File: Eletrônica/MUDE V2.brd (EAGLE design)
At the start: 35 x 16 mm, 36 parts, among them J1 22-05-7038-03, J2 22-05-7038-03, Q1 MOSFET-NCHANNEL2N7002PW, Q2 MOSFET-NCHANNEL2N7002PW, Q3 MOSFET-NCHANNEL2N7002PW, Q4 MOSFET-NCHANNEL2N7002PW, Q5 MOSFET-NCHANNEL2N7002PW, U2 Tiny85-20-SMT

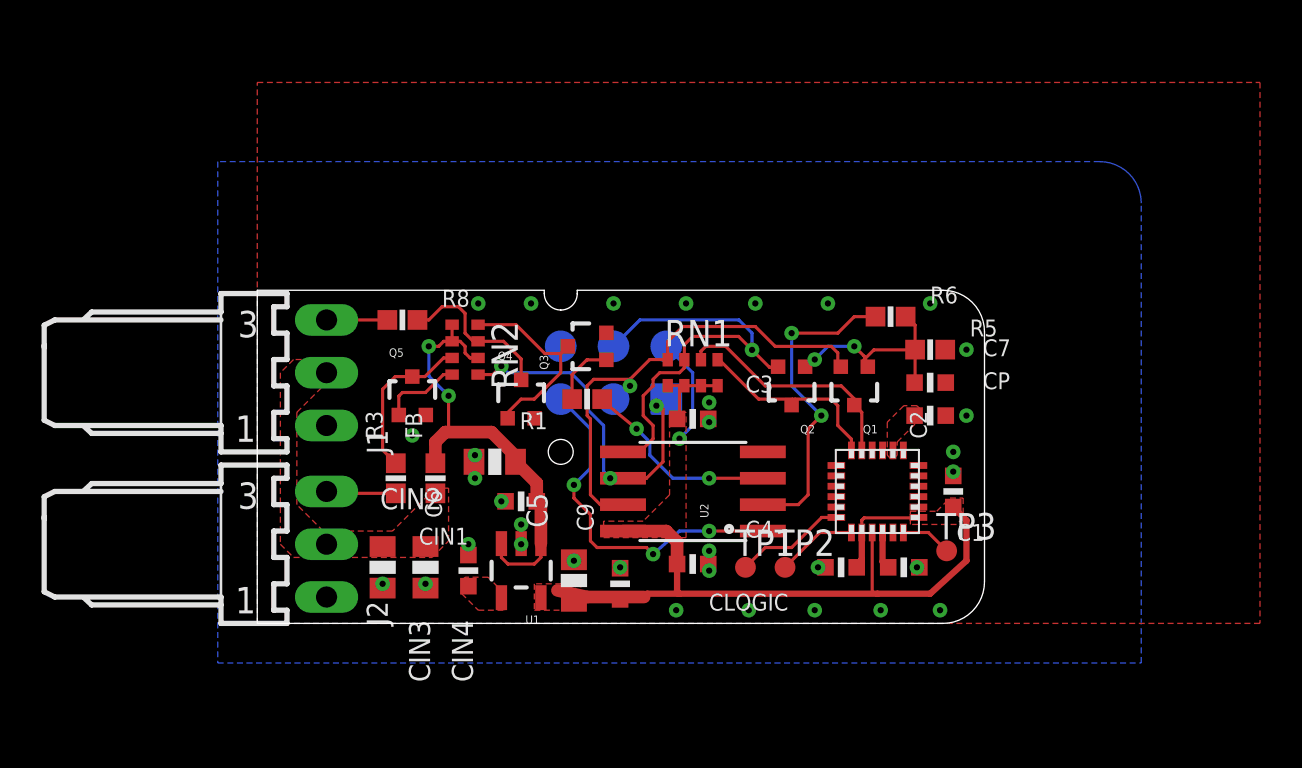
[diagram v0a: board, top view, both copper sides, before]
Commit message: MUDE V2 files
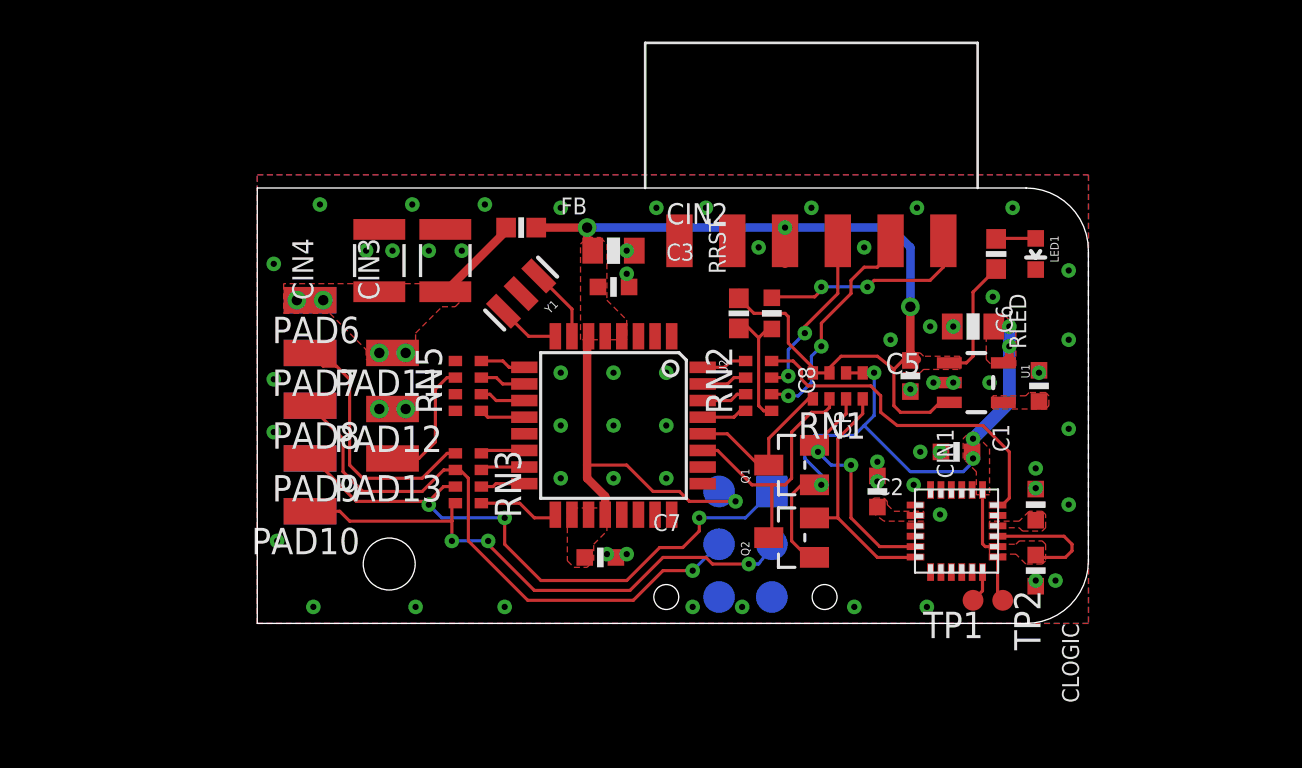
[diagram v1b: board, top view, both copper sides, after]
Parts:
- removed C4, C9: 1uF, wes:C0603
- removed J1, J2: 22-05-7038-03, con-molex:7395-03
- removed Q3, Q4, Q5: MOSFET-NCHANNEL2N7002PW, SparkFun-DiscreteSemi:SOT323
- removed R1, R3, R5, R6, R8: (no value), wes:R0603
- removed TP3: TPSQTP10R, testpad:TP10R
- added C8: 100nF, wes:C0603
- added LED1: (no value), SparkFun-LED:LED-0603
- added PAD1, PAD10, PAD11, PAD12, PAD13, PAD2, PAD3, PAD4, PAD5, PAD6, PAD7, PAD8, PAD9: (no value), wirepad:SMD1,27-2,54
- added RLED, RRST: (no value), wes:R0603
- added RN3, RN5: (no value), resistor-dil:0603-ARV
- added U$2: FTDI_HEADERSMD, wes:FTDI_HEADER_SMD
- added Y1: 16MHz, SparkFun-FreqCtrl:RESONATOR-SMD
- CIN3, CIN4: device wes:C0805 -> wes:C1210
- Q1, Q2: value MOSFET-NCHANNEL2N7002PW -> NFET; device SparkFun-DiscreteSemi:SOT323 -> SparkFun-DiscreteSemi:SOT23
- U$3: value ISP_POGOISP_LHOLE -> ISP_POGOISP_POGO; device wes:ISP_POGO_LHOLE -> wes:ISP_POGO
- U2: value Tiny85-20-SMT -> ATMEGA328P; device SparkFun-DigitalIC:SO08-EIAJ -> SparkFun-DigitalIC:TQFP32-08
- moved C6 28.9 mm to (37.6, 11.4)
- moved U1 23.7 mm to (34.6, 11.6), turned to 270 degrees
- moved C5 22.8 mm to (34.4, 14.3), turned to 180 degrees
- moved CIN1 19.7 mm to (31.4, 11.9), turned to 270 degrees
- moved C7 18.0 mm to (16.5, 3.17)
- moved CIN3 15.1 mm to (9.05, 17.5), turned to 90 degrees
- moved CIN4 14.9 mm to (5.87, 17.5), turned to 90 degrees
- moved RN2 14.2 mm to (24.1, 11.4), turned to 270 degrees
- moved FB 12.8 mm to (12.7, 19.1), turned to 0 degrees
- moved CIN2 11.7 mm to (17.1, 17.9), turned to 0 degrees
- moved TP1 11.1 mm to (34.4, 1.11), turned to 180 degrees
- moved TP2 10.6 mm to (35.9, 1.11), turned to 270 degrees
- moved U$3 10.4 mm to (23.5, 3.81), turned to 0 degrees
- moved CLOGIC 9.37 mm to (37.5, 2.54), turned to 270 degrees
- moved C3 7.41 mm to (17.1, 16.2)
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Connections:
- removed net ATTINYOUT: J2.3, R3.1
- removed net DATAOUT: R1.1, U2.3
- removed net I2C-SWITCH: R6.1, U2.2
- removed net N$17: C7.1, Q1.1, Q2.1, R5.1, R6.2
- removed net N$21: Q4.3, R8.2, RN2.3
- removed net SCL/SCK: Q1.2, RN1.4, U$3.SCK, U2.7
- removed net SDA/MOSI: Q2.2, RN1.3, U$3.MOSI, U2.5
- removed net VIN: CIN3.1, CIN4.1, FB.1, J1.2, J2.2
- new net +5V: C3.1, C7.1, CIN1.1, CIN2.1, FB.2, RLED.2, RN1.7, RN1.8, RRST.2, U$2.VCC, U$3.VCC, U1.1, U1.3, U2.18, U2.20, U2.4, U2.6
- new net DTR: C8.1, U$2.DTR
- new net MOSI: PAD8.1, RN3.6, U$3.MOSI
- new net MPU_INT: RN2.8, U$1.12
- new net N$10: U2.7, Y1.1
- new net N$15: U2.8, Y1.3
- new net N$19: RN2.4, U2.29
- new net N$20: RN5.6, U2.11
- new net N$22: RN3.1, U2.17
- new net N$23: RN3.2, U2.16
- new net N$24: RN3.3, U2.15
- new net N$25: RN3.4, U2.14
- new net N$26: RN5.5, U2.12
- new net N$29: C8.2, RN2.5, RRST.1
- new net N$30: RN5.1
- new net N$32: RN5.3
- new net N$33: RN5.4
- new net N$8: RN5.8, U2.9
- new net RX: RN2.6, U$2.RX
- new net SCK: PAD10.1, RN3.8, U$3.SCK
- new net SCL: Q1.3, RN1.1, U2.28
- new net SDA: Q2.3, RN1.2, U2.27
- new net SS: PAD7.1, RN3.5
- new net TX: RN2.7, U$2.TX
- net +3V3: now also Q1.1, Q2.1; no longer C3.1, C4.1, C9.1, RN1.7, RN1.8, U$3.VCC, U2.8
- net GND: now also LED1.C, PAD12.1, PAD2.1, PAD3.1, PAD4.1, PAD5.1, U$2.GND, U2.21, U2.3, U2.5, Y1.2; no longer C4.2, C9.2, J1.1, J2.1, Q3.2, Q4.2, Q5.2, R5.2, U2.4
- net MISO: now also PAD9.1, RN3.7; no longer RN2.1, U2.6
- net N$11: now also LED1.A, RLED.1; no longer TP3.TP, U$1.12
- net N$14: now also RN2.2, U2.31; no longer Q3.1, R1.2
- net N$16: now also RN5.7, U2.10; no longer Q3.3, Q4.1, RN2.4
- net N$18: now also RN2.1, U2.32; no longer Q5.3, R3.2, RN2.7
- net N$2: now also RN2.3, U2.30; no longer Q5.1, RN2.8
- net N$7: now also Q2.2, RN1.4; no longer Q2.3, RN1.1
- net N$9: now also Q1.2, RN1.3; no longer Q1.3, RN1.2
- net NEOPIXELS: now also PAD13.1, RN5.2; no longer J1.3, R8.1
- net RST: no longer U2.1
- net V+: now also CIN3.1, CIN4.1, FB.1, PAD1.1, PAD11.1, PAD6.1; no longer CIN1.1, CIN2.1, FB.2, RN2.2, RN2.5, RN2.6, U1.1, U1.3
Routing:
- net +5V: track 0.00 -> 68.6 mm, vias 0 -> 4
- net MOSI: track 0.00 -> 28.2 mm, vias 0 -> 1
- net SCK: track 0.00 -> 27.0 mm, vias 0 -> 3
- net SCL/SCK: track 23.7 -> 0.00 mm, vias 1 -> 0
- net SDA/MOSI: track 21.4 -> 0.00 mm, vias 1 -> 0
- net V+: track 22.1 -> 4.93 mm, vias 2 -> 4
- net RST: track 17.1 -> 0.00 mm, vias 3 -> 0
- net MPU_INT: track 0.00 -> 16.9 mm
- net I2C-SWITCH: track 15.4 -> 0.00 mm, vias 2 -> 0
- net SDA: track 0.00 -> 12.7 mm
- net SS: track 0.00 -> 12.4 mm
- net MISO: track 17.0 -> 29.2 mm
- net RX: track 0.00 -> 11.0 mm, vias 0 -> 2
- net N$17: track 10.3 -> 0.00 mm, vias 2 -> 0
- net DTR: track 0.00 -> 10.2 mm, vias 0 -> 2
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- added copper zone on layer 1, net +5V
- added copper zone on layer 1, net N$12
- added copper zone on layer 1, net V+
- removed copper zone on layer 1, net VIN
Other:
- board size 35 x 16 mm -> 40 x 21 mm
